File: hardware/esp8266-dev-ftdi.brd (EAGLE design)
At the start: 50 x 50 mm, 32 parts, among them CON1 USBMICRO-NO_CENTER

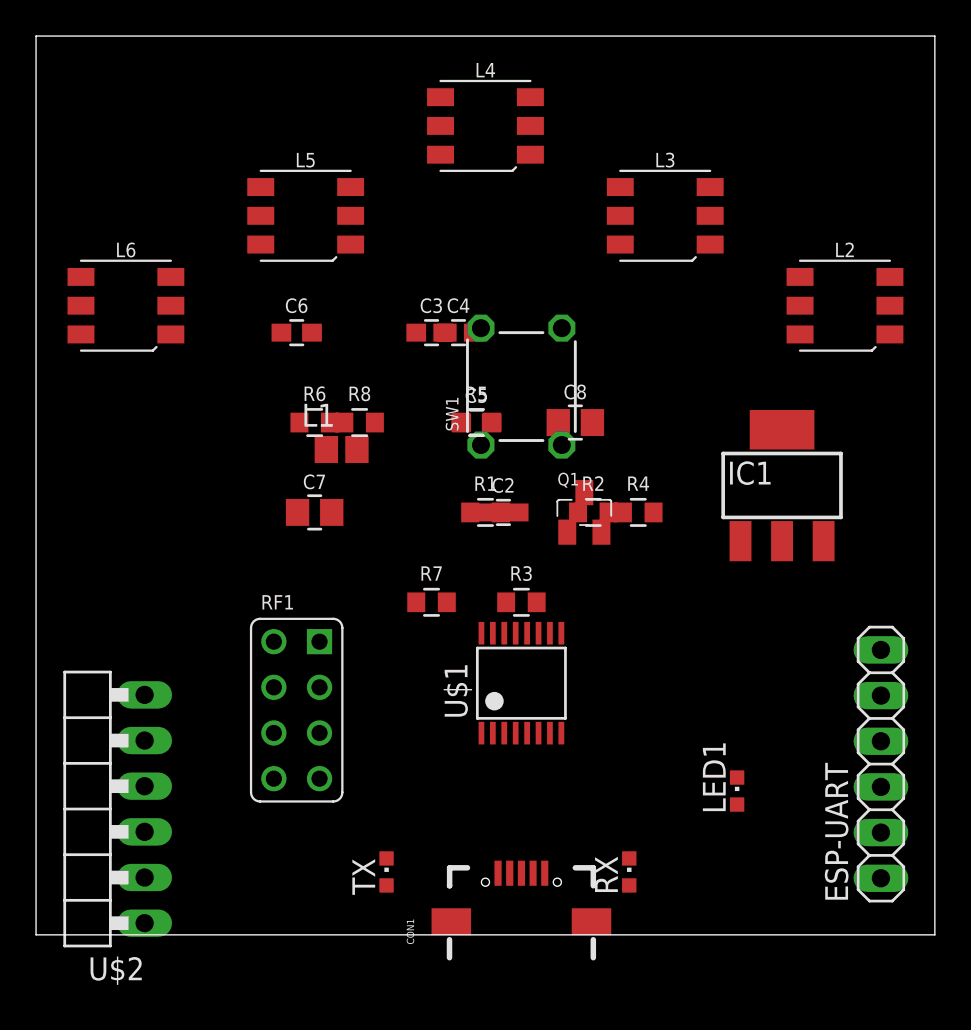
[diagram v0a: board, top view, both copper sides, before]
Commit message: schematic mostly done
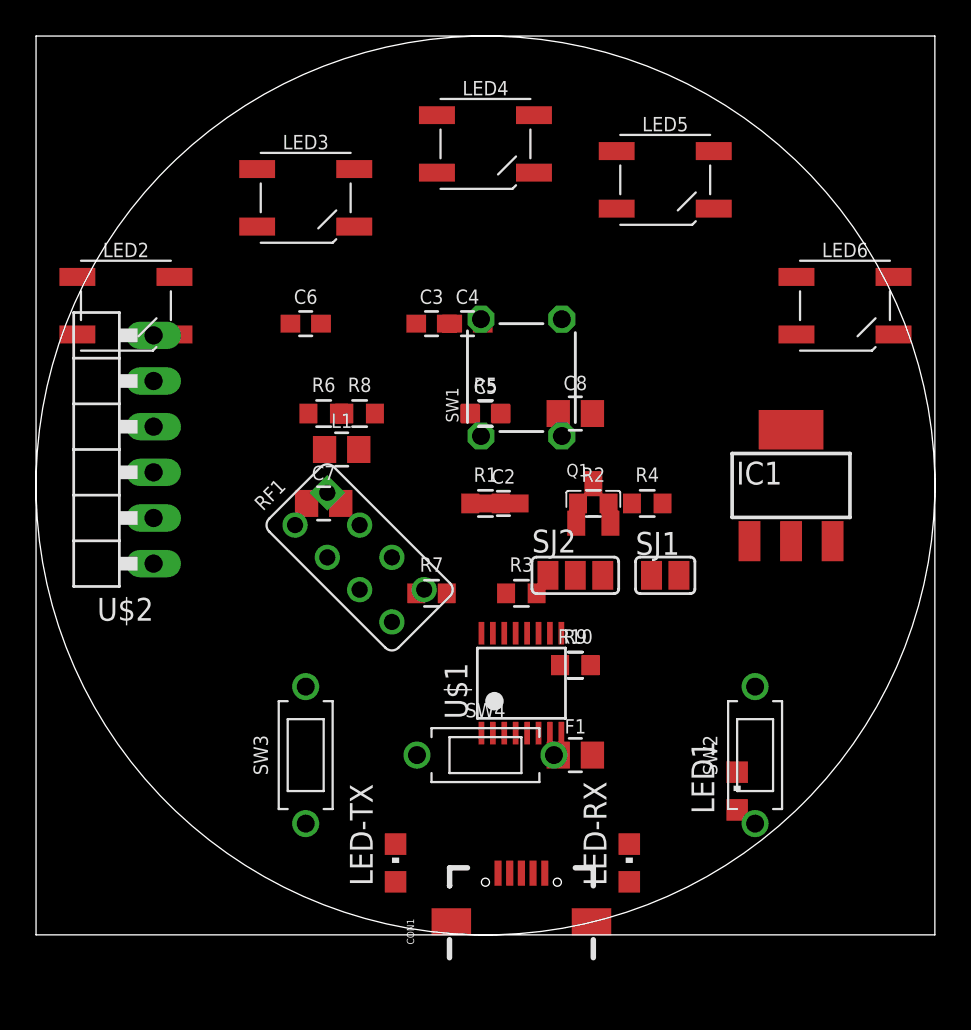
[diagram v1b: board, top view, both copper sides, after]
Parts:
- removed ESP-UART: (no value), p.peter-connectors:PINHEADER-100MIL-1X6
- removed L2, L3, L4, L5, L6: WS2812S, p.peter-leds:CHIP-5050
- removed RX, TX: (no value), p.peter-leds:CHIPLED_0603
- added F1: 500mA, p.peter-regulators:SMD-FUSE-0805
- added LED-RX, LED-TX: (no value), p.peter-leds:CHIPLED_0805
- added LED2, LED3, LED4, LED5, LED6: (no value), p.peter-leds:CHIP-5050-4_PIN
- added R10, R9: 2k, p.peter-rcl:R0603
- added SJ1: (no value), jumper:SJ
- added SJ2: (no value), jumper:SJ_2
- added SW2, SW3, SW4: (no value), p.peter-passives:SWITCH-GENERIC-2_PIN
- L1: value (none) -> 875-MI0805K601R-10; device dp_devices:FB603 -> p.peter-passives:R0805
- LED1: device p.peter-leds:CHIPLED_0603 -> p.peter-leds:CHIPLED_0805
- moved U$2 20.0 mm to (4.00, 27.0)
- moved RF1 9.19 mm to (18.0, 21.0), turned to 45 degrees
- moved C4 0.71 mm to (24.0, 34.0)
- moved C5 0.71 mm to (25.0, 29.0)
- moved C6 0.71 mm to (15.0, 34.0)
- moved C7 0.71 mm to (16.0, 24.0)
- moved Q1 0.71 mm to (31.0, 24.0)
- moved R4 0.71 mm to (34.0, 24.0)
- moved R5 0.71 mm to (25.0, 29.0)
- moved R6 0.71 mm to (16.0, 29.0)
- moved C2 0.50 mm to (26.0, 24.0)
- moved C3 0.50 mm to (22.0, 34.0)
- moved C8 0.50 mm to (30.0, 29.0)
- moved IC1 0.50 mm to (42.0, 25.0)
- moved R1 0.50 mm to (25.0, 24.0)
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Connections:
- new net N$12: LED2.P$2, LED3.P$4
- new net N$15: LED3.P$2, LED4.P$4
- new net N$16: LED4.P$2, LED5.P$4
- new net N$17: LED5.P$2, LED6.P$4
- new net N$18: CON1.VUSB, F1.2, SJ1.2
- new net N$20: R9.2, SW3.P$1
- new net N$21: R10.2, SW4.P$1
- new net VCCIO: SJ2.2, U$1.3, U$2.3
- net +3V3: now also SJ2.3; no longer ESP-UART.3, U$1.3
- net +5V: now also LED2.P$1, LED3.P$1, LED4.P$1, LED5.P$1, LED6.P$1, SJ2.1; no longer U$2.3
- net /SLEEP: now also U$2.6
- net CTS: now also U$2.2
- net GND: now also LED-RX.C, LED-TX.C, LED2.P$3, LED3.P$3, LED4.P$3, LED5.P$3, LED6.P$3, R10.1, R9.1, SW2.P$1; no longer ESP-UART.1, RX.C, TX.C
- net IO2: now also LED2.P$4
- net N$10: now also SW2.P$2
- net N$2: now also F1.1, SJ1.1; no longer CON1.VUSB
- net N$3: now also LED-TX.A; no longer TX.A
- net N$8: now also LED-RX.A; no longer RX.A
- net RX: now also SW4.P$2; no longer ESP-UART.5
- net TX: now also SW3.P$2; no longer ESP-UART.4
